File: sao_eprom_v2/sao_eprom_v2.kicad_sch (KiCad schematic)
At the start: 45 parts, among them J1 Conn_01x03, J2 USB_C_Receptacle_USB2.0, J3 sao_v2_addon_tht, J4 Conn_01x02, J5 I2C, J6 I2C, U1 W25Q128JVS, U11 W25Q16JVUXIQ, U2 RP2040, U3 24LC00, X1 SX3M12.000M20F30TNN

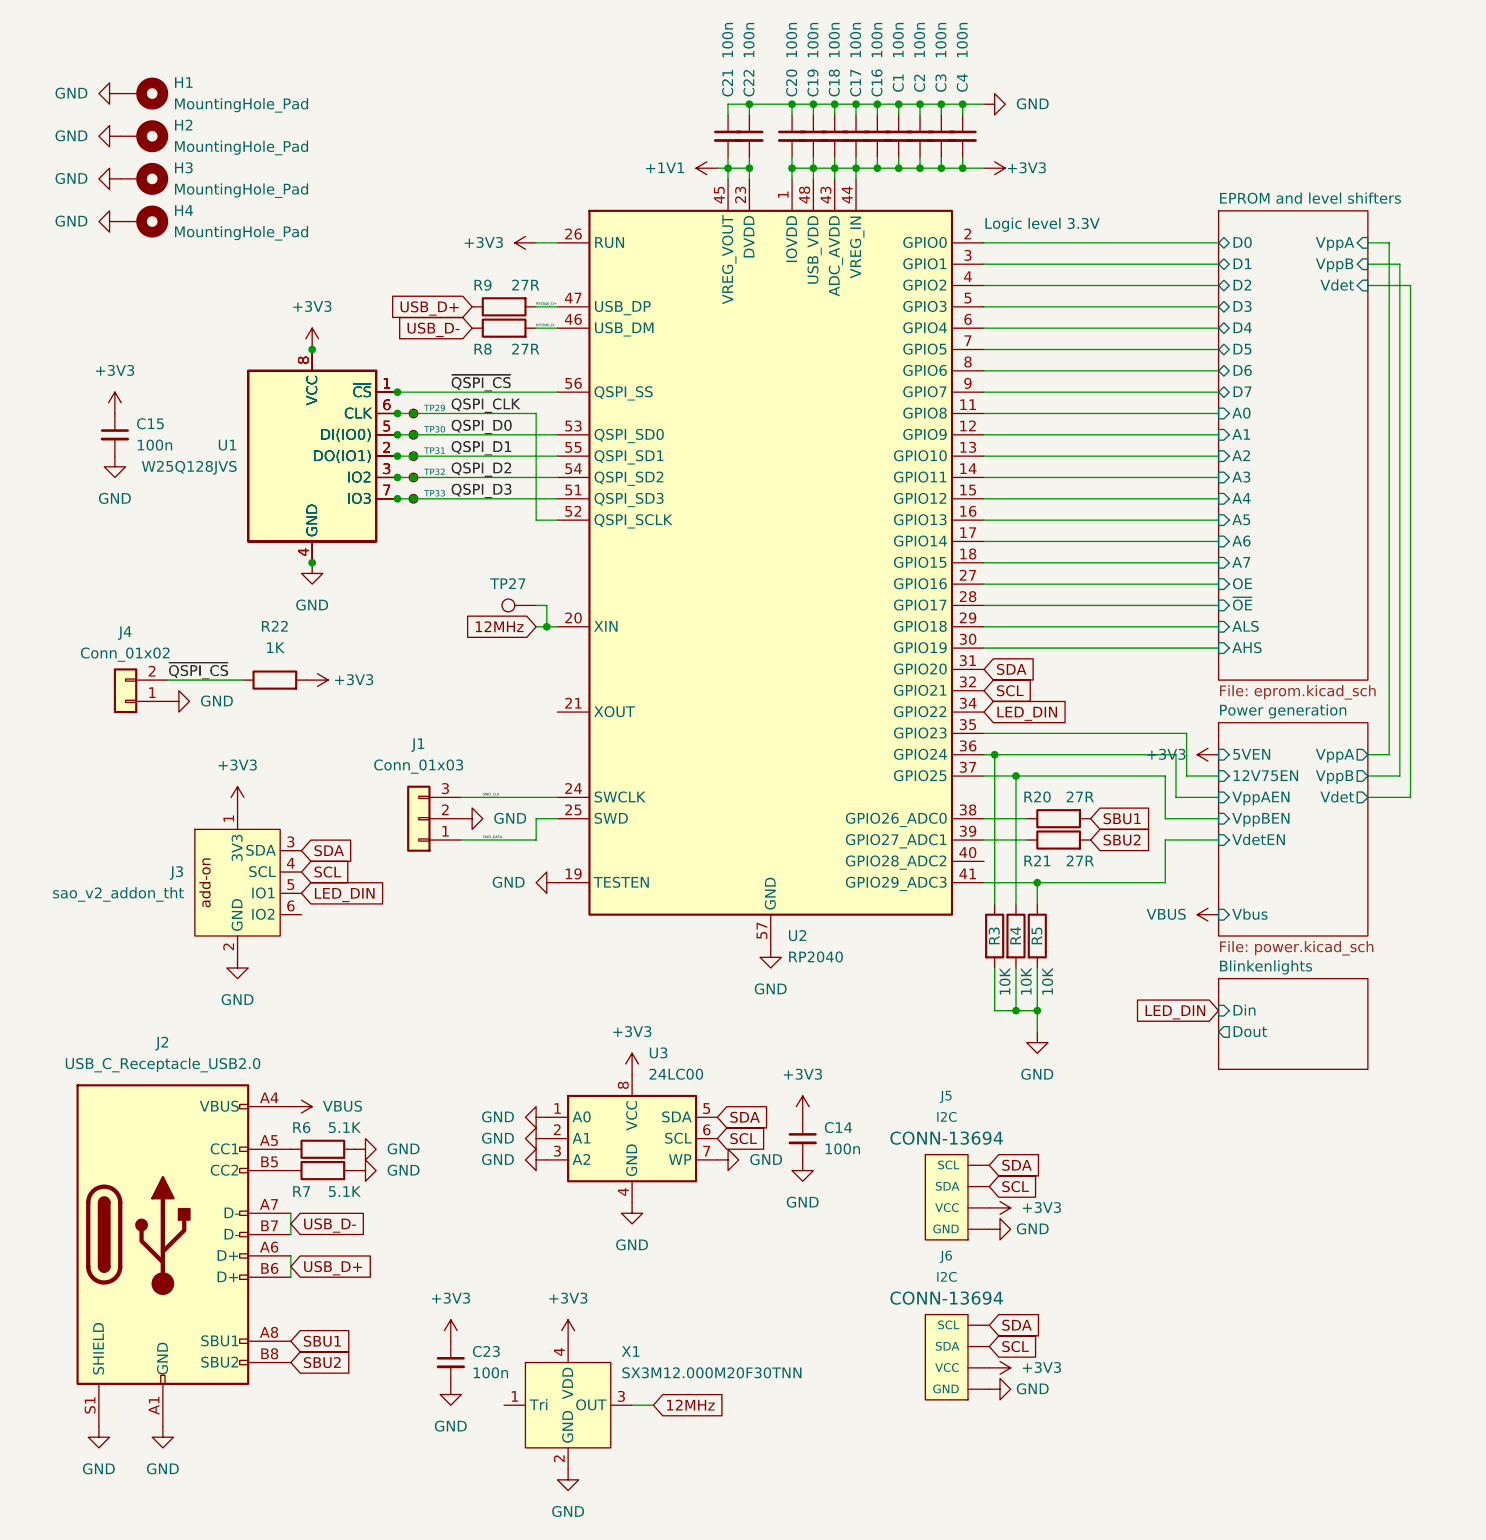
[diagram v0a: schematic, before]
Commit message: Candidate revision No. 1
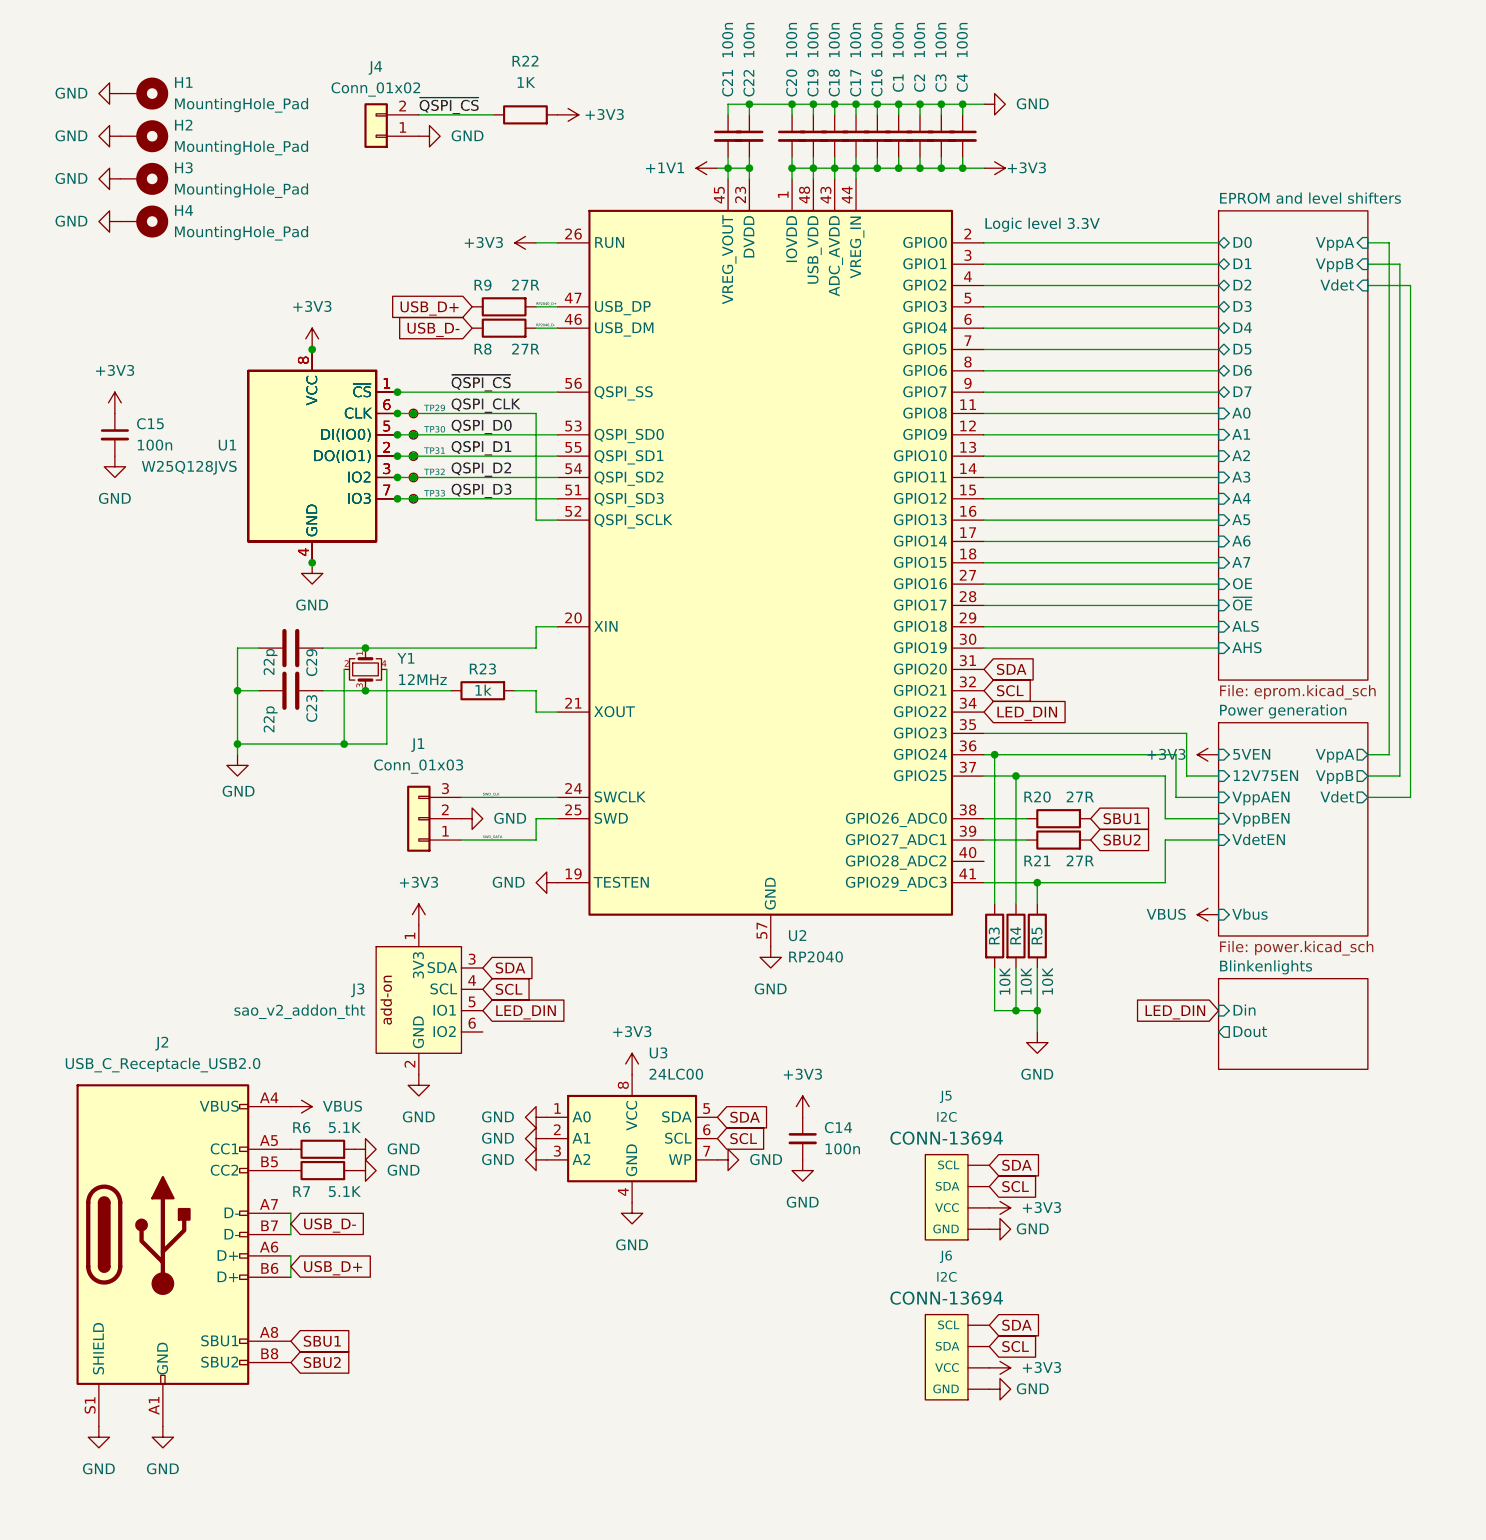
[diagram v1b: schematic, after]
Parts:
- removed C23: 100n, Capacitor_SMD:C_0402_1005Metric_Pad0.74x0.62mm_HandSolder, symbol Device:C_Small
- removed TP27: TestPoint, TestPoint:TestPoint_Pad_D1.0mm, symbol Connector:TestPoint
- removed X1: SX3M12.000M20F30TNN, Crystal:Crystal_SMD_3225-4Pin_3.2x2.5mm, symbol oscillator:YSO110TR
- added C23, C29: 22p, Capacitor_SMD:C_0402_1005Metric_Pad0.74x0.62mm_HandSolder, symbol mch2021-rescue:C-Device
- added R23: 1k, Resistor_SMD:R_0402_1005Metric_Pad0.72x0.64mm_HandSolder, symbol mch2021-rescue:R-Device
- added Y1: 12MHz, Crystal:Crystal_SMD_3225-4Pin_3.2x2.5mm, symbol mch2021-rescue:Crystal_GND24_Small-Device
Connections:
- net GND: now also C23.2, C29.2, Y1.2, Y1.4
- net at U2.21 (XOUT): now also R23.2
- net 12MHz: no longer names the net of U2.20 (XIN)
- net 12MHz: now also C29.1, Y1.1
- new net: C23.1, R23.1, Y1.3
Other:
- moved on the sheet: J3, J4, R22
